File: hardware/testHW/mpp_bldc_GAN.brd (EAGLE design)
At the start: 36.5 x 20.4 mm, 67 parts, among them IC1 ATXMEGA16A4U-MH, U1 LM3480IM3-5, U3 MIC5504-2.8YM5-TR, X1 PASSER-07, X2 PASSER-07, X3 PASSER-07, X4 PASSER-07

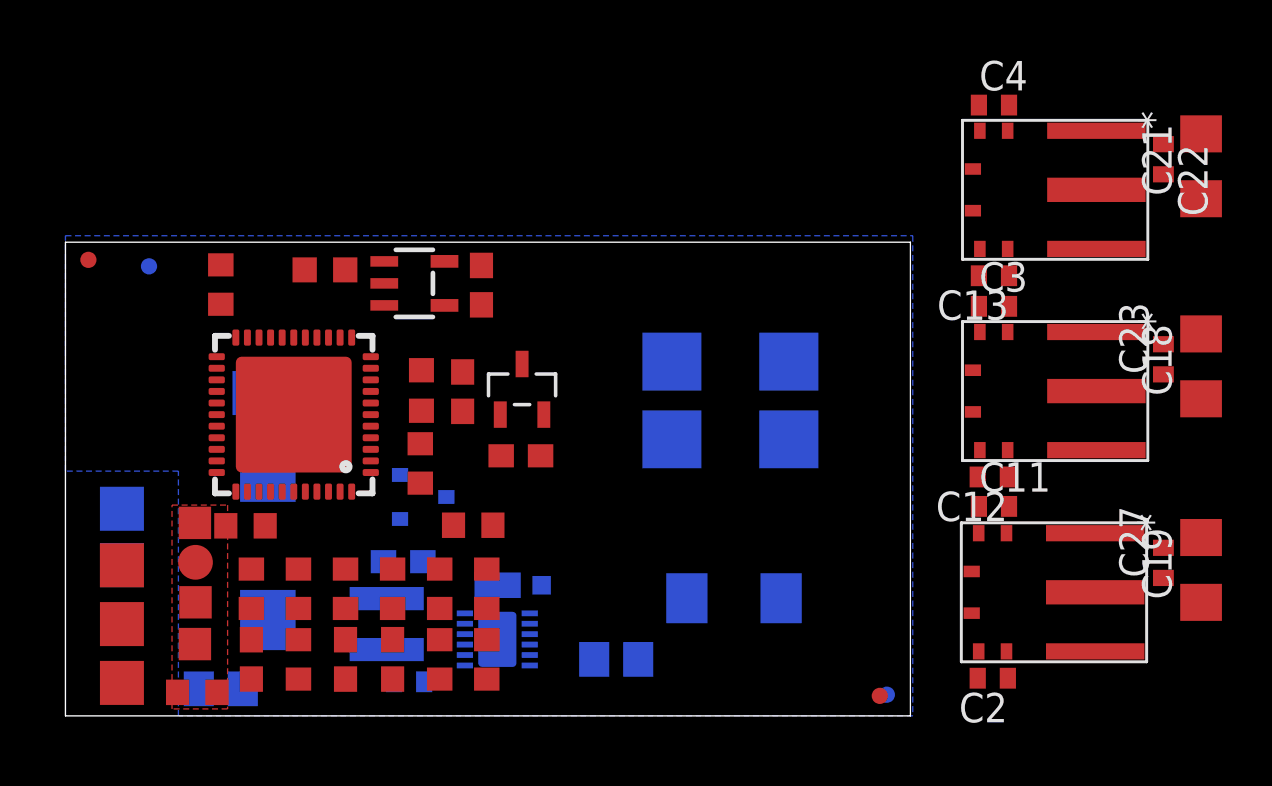
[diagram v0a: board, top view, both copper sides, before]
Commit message: testing
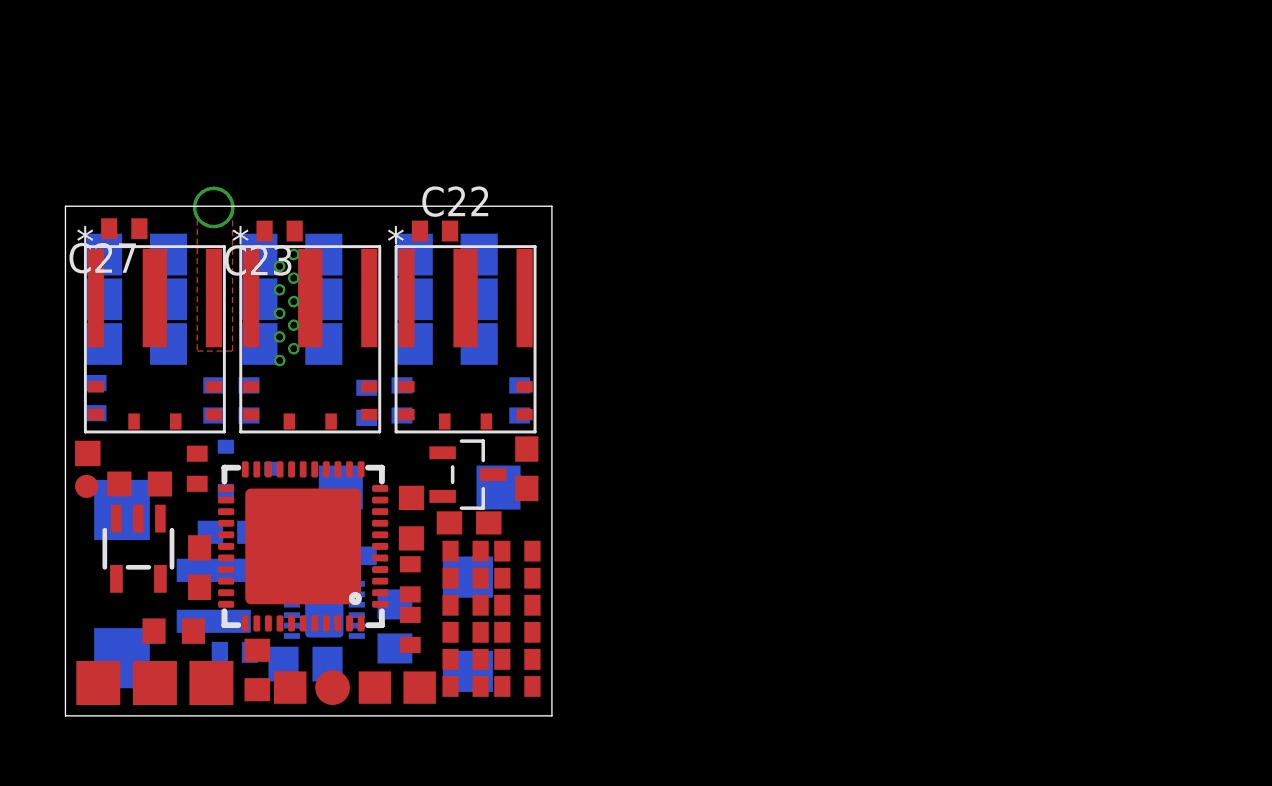
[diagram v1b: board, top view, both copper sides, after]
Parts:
- removed C16, C17: CAP TANT 22UF 25V 10% 2312, rcl:C/6032-28R
- removed X1, X2, X3, X4: PASSER-07, we-symbol:PASSER_07MM
- added C1, C28, C29, C30, C31, C32: 10uF/25V/CC, rcl:C1206
- C5, C6, C7: device rcl:C0603 -> rcl:C0402
- R12, R13, R14, R15, R16, R17, R18, R19, R20, R21, R22: device rcl:R0603 -> rcl:R0402
- R2: device resistor:R0603 -> resistor:R0402
- RX_DIRECT: value TPSQTP19SQ -> TPSQTP11SQ; device testpad:TP19SQ -> testpad:TP11SQ
- TP7: value TPSQTP19SQ -> TPSQTP10R; device testpad:TP19SQ -> testpad:TP10R
- moved C27 47.1 mm to (2.54, 21.0), turned to 180 degrees
- moved C19 47.0 mm to (3.05, 16.1), flipped to the bottom, turned to 0 degrees
- moved U$1 40.3 mm to (3.86, 16.3), turned to 0 degrees
- moved C18 39.4 mm to (9.75, 18.0), flipped to the bottom, turned to 0 degrees
- moved C11 39.0 mm to (1.32, 13.7), flipped to the bottom, turned to 90 degrees
- moved C23 38.6 mm to (9.25, 20.9), turned to 180 degrees
- moved C2 35.7 mm to (6.40, 13.6), flipped to the bottom, turned to 270 degrees
- moved C21 33.5 mm to (16.5, 16.1), flipped to the bottom, turned to 0 degrees
- moved C3 32.4 mm to (7.92, 13.6), flipped to the bottom, turned to 90 degrees
- moved U$2 32.2 mm to (10.6, 16.3), turned to 0 degrees
- moved C22 31.6 mm to (16.0, 20.9), turned to 0 degrees
- moved C4 28.6 mm to (14.5, 13.6), flipped to the bottom, turned to 90 degrees
- moved C12 27.2 mm to (13.0, 13.5), flipped to the bottom, turned to 270 degrees
- moved U$3 26.3 mm to (17.3, 16.3), turned to 0 degrees
- moved C13 21.2 mm to (19.6, 13.6), flipped to the bottom, turned to 270 degrees
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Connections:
- net N$1 renamed PROG_JMP
- removed net RC_SIG_IC: IC1.4, R1.2
- new net N$4: IC1.32, R1.2
- net GND: now also C1.1, C28.1, C29.1, C30.1, C31.1, C32.1; no longer C16.-, C17.-
- net VCC: now also C1.2, C28.2, C29.2, C30.2, C31.2, C32.2; no longer C16.+, C17.+
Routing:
- added copper zone on layer 1, net W
- removed copper zone on layer 2, net +3V3
- removed copper zone on layer 2, net +5V
- removed copper zone on layer 1, net GND
- removed copper zone on layer 15, net GND
- removed copper zone on layer 16, net GND
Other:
- board size 36.5 x 20.4 mm -> 21 x 22 mm
- board text removed: "+"
- board text removed: "-"
